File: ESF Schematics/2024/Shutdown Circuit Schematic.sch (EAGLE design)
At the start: 32 parts, among them J1 CONNECTOR-1_6MM2, J10 CONNECTOR-1_CT2242-2, J11 CONNECTOR-3_XXC106-EV-P3Z, J15 CONNECTOR-3_NEMA-5-20, J16 CONNECTOR-3_NEMA-5-20, J17 CONNECTOR-2_, J18 CONNECTOR-2_, J2 CONNECTOR-1_LCAX2-14F-E, J3 CONNECTOR-1_6MM2, J4 CONNECTOR-1_LCAX2-14F-E, J5 CONNECTOR-3_XXC106-EV-P3Z, J6 RING_TERMINAL_19054-0042, J7 RING_TERMINAL_19054-0042, J8 CONNECTOR-3_NEMA-5-20, J9 CONNECTOR-1_CT2242-2

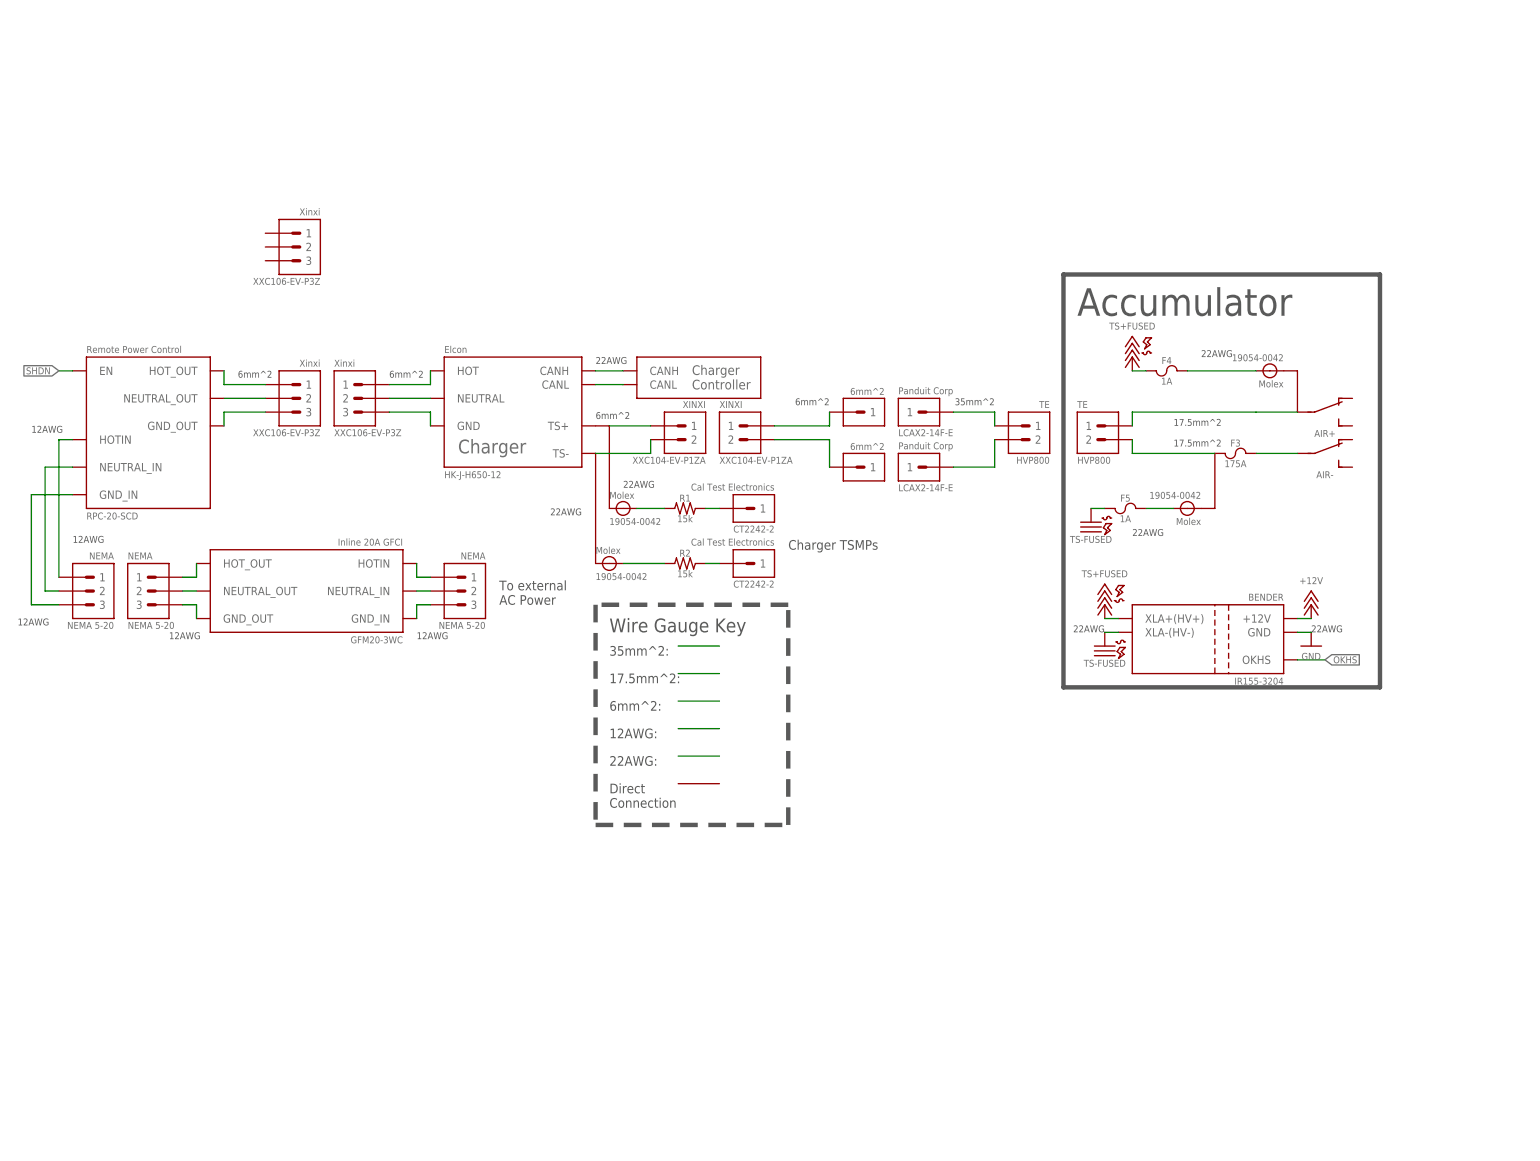
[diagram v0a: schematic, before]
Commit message: num num
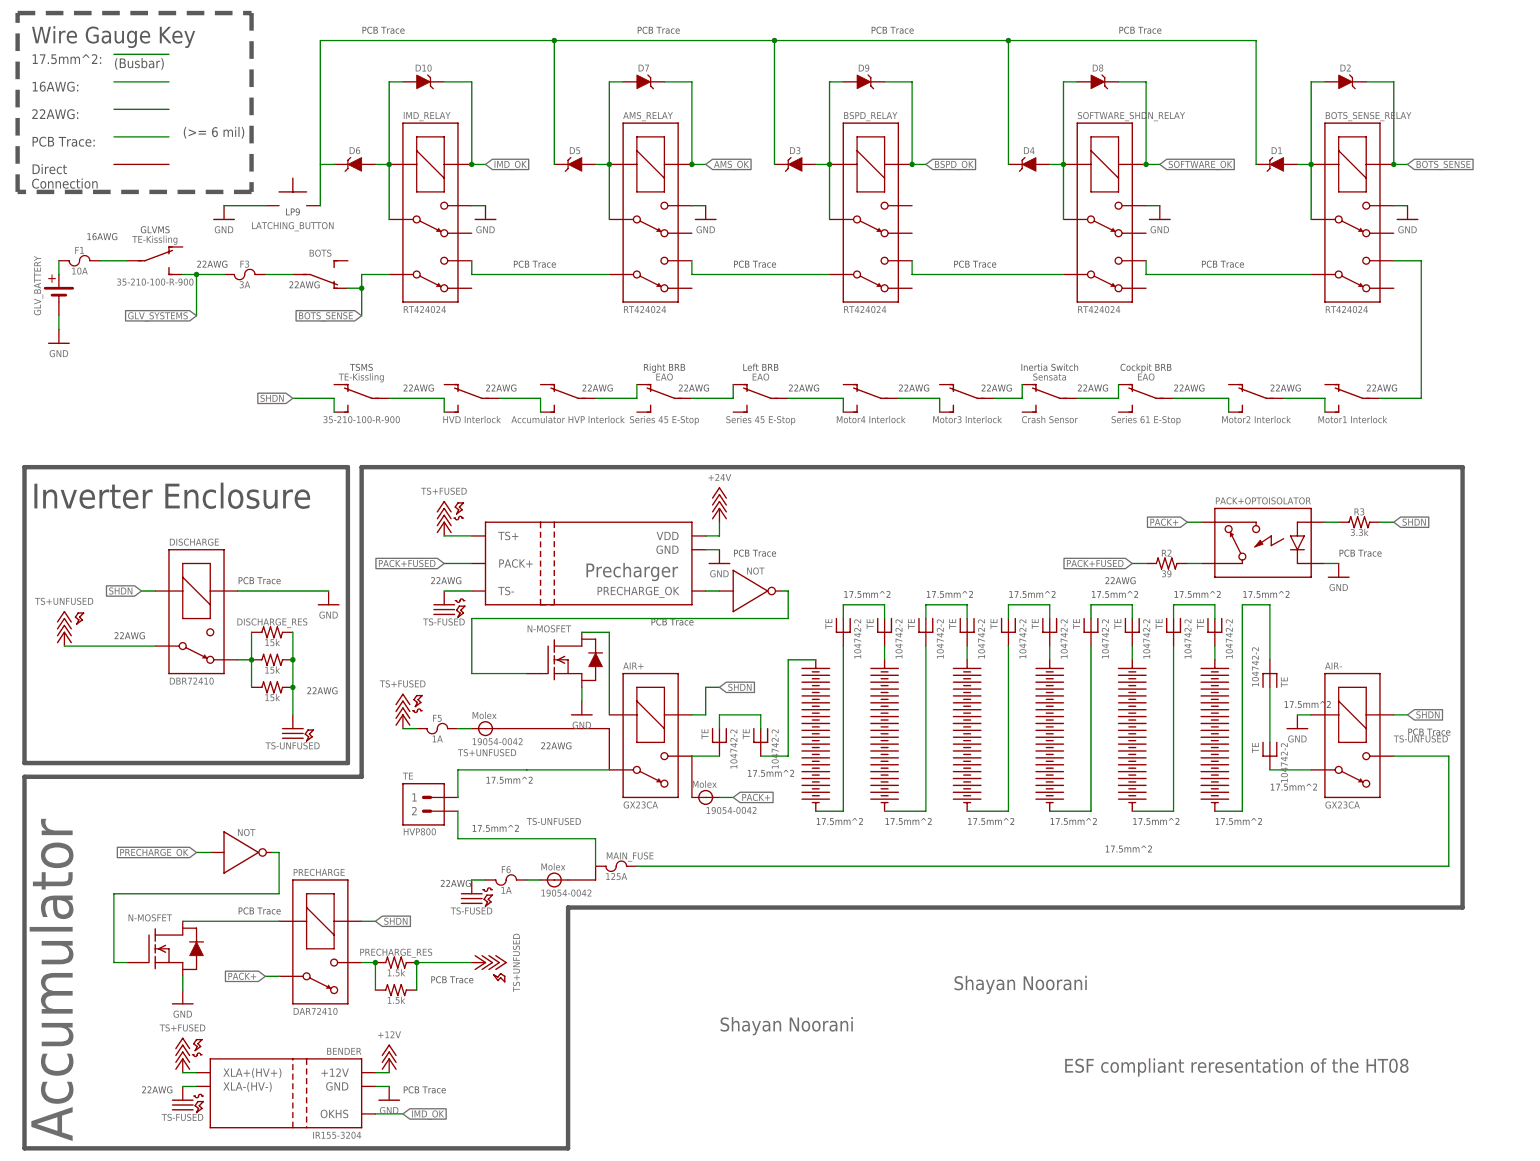
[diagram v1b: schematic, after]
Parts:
- removed A1: REMOTE_POWER_CONTROL_RPC-20-SCD, HyTechSymbolsTemp:REMOTE_POWER_CONTROL_RPC-20-SCD
- removed A2: CHARGER_HK-J-H650-12, HyTechSymbols:CHARGER_HK-J-H650-12
- removed A3: INLINE_GFCI_GFM20-3WC, HyTechSymbolsTemp:INLINE_GFCI_GFM20-3WC
- removed F4: 1A, HyTechSymbolsTemp:FUSE
- removed J10, J9: CONNECTOR-1_CT2242-2, HyTechSymbolsTemp:CONNECTOR-1_CT2242-2
- removed J11, J5: CONNECTOR-3_XXC106-EV-P3Z, HyTechSymbols:CONNECTOR-3_XXC106-EV-P3Z
- removed J15, J16, J8: CONNECTOR-3_NEMA-5-20, HyTechSymbolsTemp:CONNECTOR-3_NEMA-5-20
- removed J17, J18: CONNECTOR-2_, HyTechSymbols:CONNECTOR-2_XXC104-EV-P1ZA
- removed J2, J4: CONNECTOR-1_LCAX2-14F-E, HyTechSymbols:CONNECTOR-1_LCAX2-14F-E
- removed J3: CONNECTOR-1_6MM2, HyTechSymbols:CONNECTOR-1_6MM2
- removed J6, J7: RING_TERMINAL_19054-0042, HyTechSymbols:RING_TERMINAL_19054-0042
- removed R1: 15k, HyTechSymbolsTemp:RESISTOR
- removed U$7: RING_TERMINAL_19054-0042, HyTechSymbolsTemp:RING_TERMINAL_19054-0042
- added AIR+, AIR-: RELAY_SPST_NO_, HyTechSymbols:RELAY_SPST_NO_
- added AMS_RELAY, BOTS_SENSE_RELAY, BSPD_RELAY, IMD_RELAY, SOFTWARE_SHDN_RELAY: RELAY_DPDT_RT424024, HyTechSymbols:RELAY_DPDT_RT424024
- added D1, D10, D2, D3, D4, D5, D6, D7, D8, D9: DIODE, HyTechSymbolsTemp:DIODE
- added DISCHARGE: RELAY_SPST_NC_DBR72410, HyTechSymbols:RELAY_SPST_NC_DBR72410
- added DISCHARGE_RES, DISCHARGE_RES1, DISCHARGE_RES2: 15k, HyTechSymbolsTemp:RESISTOR
- added F1: 10A, HyTechSymbolsTemp:FUSE
- added F6: 1A, HyTechSymbolsTemp:FUSE
- added GLV_BATTERY: BATTERY, HyTechSymbols:BATTERY
- added LATCHING_BUTTON: BUTTON_NO_LP9, HyTechSymbolsTemp:BUTTON_NO_LP9
- added MAIN_FUSE: 125A, HyTechSymbolsTemp:FUSE
- added PACK+OPTOISOLATOR: RELAY_SOLIDSTATE_NO_, HyTechSymbolsTemp:RELAY_SOLIDSTATE_NO_
- added PRECHARGE: RELAY_SPST_NO_DAR72410, HyTechSymbols:RELAY_SPST_NO_DAR72410
- added PRECHARGE_RES, PRECHARGE_RES1: 1.5k, HyTechSymbolsTemp:RESISTOR
- added Q1, Q2: MOSFET_N-CHANNEL, HyTechSymbolsTemp:MOSFET_N-CHANNEL
- added R3: 3.3k, HyTechSymbolsTemp:RESISTOR
- added S10, S11, S12, S13, S6, S7: SWITCH_SPST_, HyTechSymbols:SWITCH_SPST_
- added S3: SWITCH_SPST_27MM_STOP, HyTechSymbols:SWITCH_SPST_27MM_STOP
- added S4, S5: SWITCH_SPST_40MM_STOP, HyTechSymbols:SWITCH_SPST_40MM_STOP
- added S8, S9: SWITCH_SPST_35-210-100-R-900, HyTechSymbols:SWITCH_SPST_35-210-100-R-900
- added U$10: BENDER_IR155-3204, HyTechSymbols:BENDER_IR155-3204
- added U$12, U$13, U$14: SEGMENT, HyTechSymbols:SEGMENT
- added U$17: PRECHARGER, HyTechSymbolsTemp:PRECHARGER
- added U$2, U$20, U$21, U$22, U$23, U$24, U$25, U$34, U$35, U$36, U$37: MAINTENANCE_PLUG_104742-2, HyTechSymbolsTemp:MAINTENANCE_PLUG_104742-2
- added U$38, U$39, U$40: RING_TERMINAL_19054-0042, HyTechSymbolsTemp:RING_TERMINAL_19054-0042
- added U1, U2: LOGICGATE_INVERTER, HyTechSymbolsTemp:LOGICGATE_INVERTER
- F3: value 175A -> 3A
- J1: value CONNECTOR-1_6MM2 -> CONNECTOR-2_HVP800; device HyTechSymbols:CONNECTOR-1_6MM2 -> HyTechSymbols:CONNECTOR-2_HVP800
- R2: value 15k -> 39
- S1: value SWITCH_SPST_ -> SWITCH_SPST_INERTIA_SWITCH; device HyTechSymbols:SWITCH_SPST_ -> HyTechSymbols:SWITCH_SPST_INERTIA_SWITCH; MPN AIR+ -> (none)
- S2: MPN AIR- -> BOTS
- U$1, U$4: value CONNECTOR-2_HVP800 -> SEGMENT; device HyTechSymbols:CONNECTOR-2_HVP800 -> HyTechSymbols:SEGMENT
- U$15: value CHARGER_CONTROLLER -> SEGMENT; device HyTechSymbolsTemp:CHARGER_CONTROLLER -> HyTechSymbols:SEGMENT
- U$3: value CONNECTOR-3_XXC106-EV-P3Z -> MAINTENANCE_PLUG_104742-2; device HyTechSymbols:CONNECTOR-3_XXC106-EV-P3Z -> HyTechSymbolsTemp:MAINTENANCE_PLUG_104742-2
- U$5: value BENDER_IR155-3204 -> MAINTENANCE_PLUG_104742-2; device HyTechSymbols:BENDER_IR155-3204 -> HyTechSymbolsTemp:MAINTENANCE_PLUG_104742-2
- U$6: value RING_TERMINAL_19054-0042 -> MAINTENANCE_PLUG_104742-2; device HyTechSymbolsTemp:RING_TERMINAL_19054-0042 -> HyTechSymbolsTemp:MAINTENANCE_PLUG_104742-2
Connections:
- removed net CHARGER_CONTROLLER_CANH: A2.CANH, U$15.CANH
- removed net CHARGER_CONTROLLER_CANL: A2.CANL, U$15.CANL
- removed net N$22 (its old number): A1.HOTIN, J15.1
- removed net N$27: R2.1, U$6.P$2
- removed net N$28: A3.HOT_OUT, J8.1
- removed net N$30: A3.GND_IN, J16.3
- removed net OKHS: U$5.OKHS
- new net +5V: U$17.VDD
- new net AMS_OK: AMS_RELAY.COIL+, D7.C
- new net BOTS_SENSE: BOTS_SENSE_RELAY.COIL+, D2.C, IMD_RELAY.6, S2.O
- new net BSPD_OK: BSPD_RELAY.COIL+, D9.C
- new net GLV_SYSTEMS: F3.1, S9.S
- new net IMD_OK: D10.C, IMD_RELAY.COIL+, U$10.OKHS
- new net N$12: S4.O, S5.P
- new net N$13: S5.O, S7.P
- new net N$16: BOTS_SENSE_RELAY.3, BOTS_SENSE_RELAY.COIL-, D1.A, D2.A
- new net N$17: S12.P, S13.S
- new net N$18: S1.O, S11.P
- new net N$34: U$14.+, U$23.1
- new net N$36: U$15.+, U$25.1
- new net N$37: U$34.P$1, U$35.P$1
- new net N$38: AIR+.CONTACT2, U$34.1
- new net N$39: PACK+OPTOISOLATOR.CONTROL+, R3.1
- new net N$40: PACK+OPTOISOLATOR.CONTACT1, R2.2
- new net N$42: BSPD_RELAY.5, SOFTWARE_SHDN_RELAY.6
- new net N$43: U$20.P$1, U$21.P$1
- new net N$44: U$22.P$1, U$23.P$1
- new net N$45: U$24.P$1, U$25.P$1
- new net N$46: U$36.P$1, U$37.P$1
- new net N$47: AIR-.CONTACT1, U$37.1
- new net N$48: F6.2, U$38.P$1
- new net N$50: F5.2, U$39.P$1
- new net N$51: S6.P, S7.S
- new net N$52: Q2.G, U2.!IN
- new net N$53: AIR+.COIL+, Q2.D
- new net N$54: U$1.+, U$3.1
- new net N$55: U$2.P$1, U$3.P$1
- new net N$56: U$36.1, U$4.-
- new net N$57: U$4.+, U$6.1
- new net N$58: U$5.P$1, U$6.P$1
- new net N$59: S12.S, S3.P
- new net PACK+: PACK+OPTOISOLATOR.CONTACT2, PRECHARGE.CONTACT1, U$12.+, U$35.1, U$40.P$2
- new net PACK+FUSED: R2.1, U$17.PACK+
- new net PRECHARGE_OK: PRECHARGE.COIL+, Q1.D, U1.IN
- new net SOFTWARE_OK: D8.C, SOFTWARE_SHDN_RELAY.COIL+
- new net TS+UNFUSED: AIR+.CONTACT1, DISCHARGE.CONTACT1, J1.1, PRECHARGE_RES.2, PRECHARGE_RES1.2
- net +12V: now also U$10.+12V; no longer U$5.+12V
- net GND: now also AIR-.COIL+, AMS_RELAY.4, BOTS_SENSE_RELAY.4, DISCHARGE.COIL-, GLV_BATTERY.P$2, IMD_RELAY.4, LATCHING_BUTTON.P$1, PACK+OPTOISOLATOR.CONTROL-, Q1.S, Q2.S, SOFTWARE_SHDN_RELAY.4, U$10.GND, U$17.GND; no longer U$5.GND
- net N$1: now also D10.A, D6.A, IMD_RELAY.3, IMD_RELAY.COIL-; no longer A2.NEUTRAL, U$3.2
- net N$10: now also AMS_RELAY.5, BSPD_RELAY.6; no longer S1.P, U$1.1
- net N$11: now also AMS_RELAY.6, IMD_RELAY.5; no longer F3.1, U$1.2
- net N$14: now also F1.1, GLV_BATTERY.P$1; no longer J1.1, J18.1
- net N$15: now also BOTS_SENSE_RELAY.6, SOFTWARE_SHDN_RELAY.5; no longer J18.2, J3.1
- net N$19: now also BOTS_SENSE_RELAY.5, S13.P; no longer A1.GND_OUT, J5.3
- net N$2: now also D1.C, D3.C, D4.C, D5.C, D6.C, LATCHING_BUTTON.P$2; no longer A2.GND, U$3.3
- net N$20: now also S10.P, S11.S; no longer J4.1, U$4.2
- net N$21: now also S6.S, S8.P; no longer J2.1, U$4.1
- net N$23: now also U$1.-, U$5.1; no longer A3.NEUTRAL_OUT, J8.2
- net N$24: now also Q1.G, U1.!IN; no longer A1.NEUTRAL_IN, J15.2
- net N$25: now also U$17.PRECHARGE_OK, U2.IN; no longer R1.1, U$7.P$2
- net N$26: now also PRECHARGE.CONTACT2, PRECHARGE_RES.1, PRECHARGE_RES1.1; no longer F5.2, J7.P$2
- net N$29: now also DISCHARGE.CONTACT2, DISCHARGE_RES.1, DISCHARGE_RES1.1, DISCHARGE_RES2.1; no longer A3.GND_OUT, J8.3
- net N$3: now also AMS_RELAY.3, AMS_RELAY.COIL-, D5.A, D7.A; no longer A2.HOT, U$3.1
- net N$31: now also U$12.-, U$20.1; no longer A3.NEUTRAL_IN, J16.2
- net N$32: now also U$13.+, U$21.1; no longer A3.HOTIN, J16.1
- net N$33: now also U$13.-, U$22.1; no longer A1.GND_IN, J15.3
- net N$35: now also U$14.-, U$24.1; no longer F4.2, J6.P$2
- net N$4: now also S10.S, S4.P; no longer J17.1
- net N$5: now also D4.A, D8.A, SOFTWARE_SHDN_RELAY.3, SOFTWARE_SHDN_RELAY.COIL-; no longer A2.TS-, J17.2
- net N$6: now also BSPD_RELAY.3, BSPD_RELAY.COIL-, D3.A, D9.A; no longer A1.HOT_OUT, J5.1
- net N$7: now also F1.2, S9.P; no longer A1.NEUTRAL_OUT, J5.2
- net N$8: now also S1.P, S3.O; no longer J9.1, R1.2
- net N$9: now also U$15.-, U$2.1; no longer J10.1, R2.2
- net SHDN: now also AIR+.COIL-, AIR-.COIL-, DISCHARGE.COIL+, PRECHARGE.COIL-, R3.2, S8.S; no longer A1.EN
- net TS+: now also F5.1, U$10.XLA+(HV+), U$17.TS+; no longer F4.1, U$5.XLA+(HV+)
- net TS-UNFUSED: now also AIR-.CONTACT2, DISCHARGE_RES.2, DISCHARGE_RES1.2, DISCHARGE_RES2.2, F6.1, J1.2, MAIN_FUSE.1, MAIN_FUSE.2, U$10.XLA-(HV-), U$17.TS-; no longer F5.1, U$5.XLA-(HV-)
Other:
- note added: "(>= 6 mil)"
- note added: "(Busbar)"
- note added: "16AWG"
- note added: "16AWG:"
- note added: "Cockpit BRB"
- note added: "ESF compliant reresentation of the HT08"
- note added: "GLVMS"
- note added: "Inertia Switch"
- note added: "Inverter Enclosure"
- note added: "Left BRB"
- note added: "PCB Trace"
- note added: "PCB Trace:"
- note added: "Right BRB"
- note added: "Shayan Noorani"
- note added: "TSMS"
- note removed: "12AWG"
- note removed: "12AWG:"
- note removed: "35mm^2"
- note removed: "35mm^2:"
- note removed: "6mm^2"
- note removed: "6mm^2:"
- note removed: "Charger TSMPs"
- note removed: "To external AC Power"
- moved on the sheet: F3, F5, R2
